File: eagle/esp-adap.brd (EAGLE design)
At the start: 26.5 x 11.2 mm, 3 parts

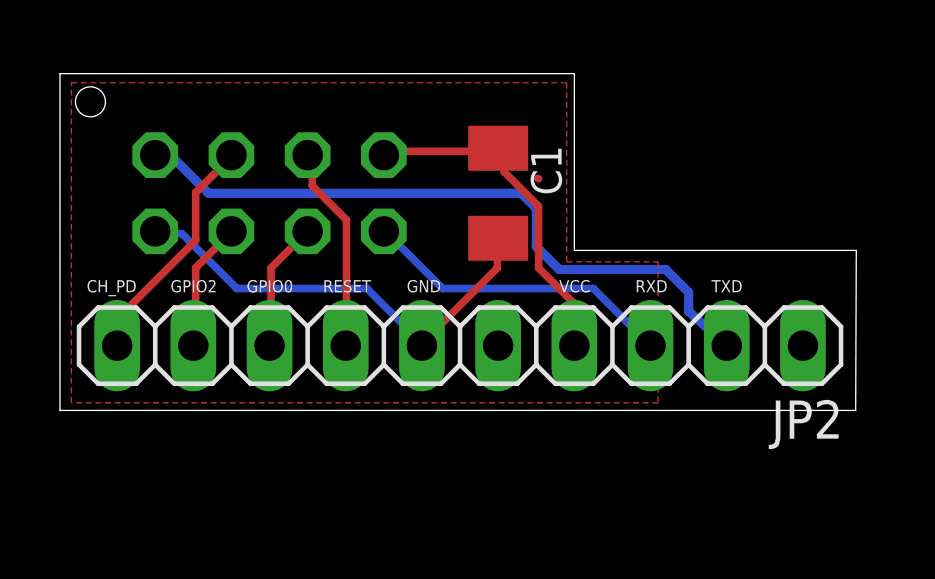
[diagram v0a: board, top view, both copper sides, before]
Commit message: added docs
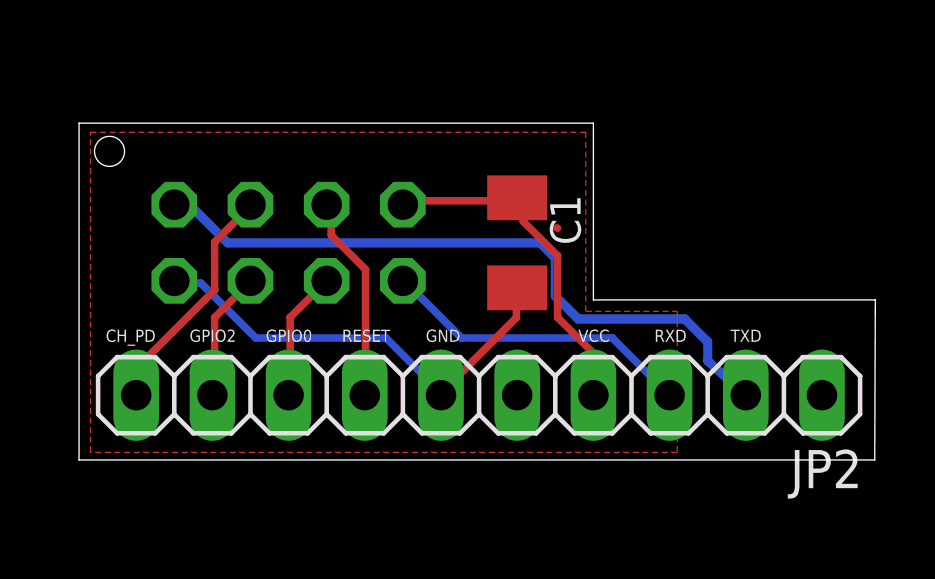
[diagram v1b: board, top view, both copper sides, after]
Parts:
- moved JP1 1.77 mm to (6.99, 7.24)
- moved JP2 1.77 mm to (13.3, 2.16)
- moved C1 1.77 mm to (14.6, 7.24)

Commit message: redefined board
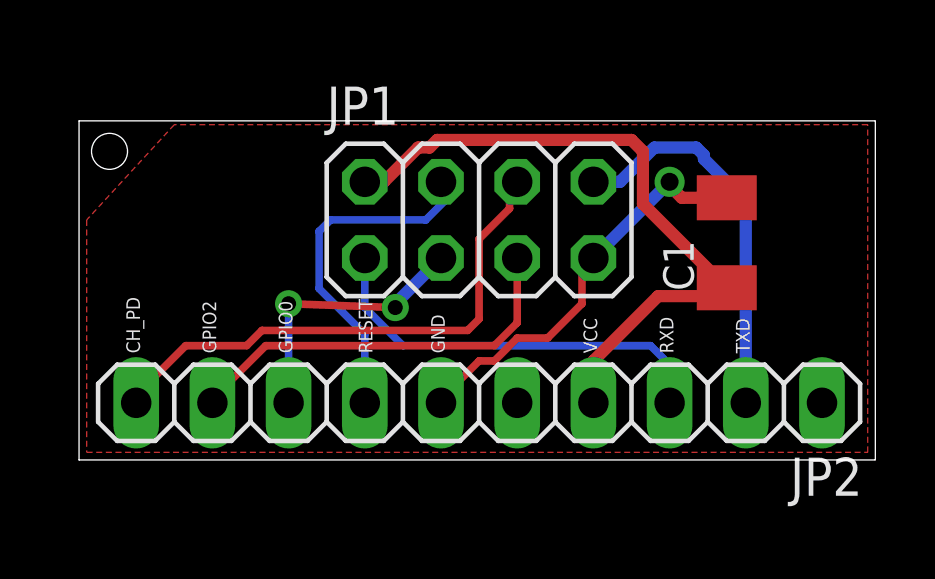
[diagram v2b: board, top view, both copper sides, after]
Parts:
- moved C1 6.98 mm to (21.6, 7.24), turned to 90 degrees
- moved JP1 6.40 mm to (13.3, 8.00), flipped to the top
- moved JP2 0.25 mm to (13.3, 1.91)
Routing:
- net VCC: track 11.6 -> 22.6 mm
- net CH_PD: track 7.93 -> 17.8 mm
- net TXD: track 22.8 -> 13.1 mm
- net GPIO2: track 4.33 -> 13.5 mm
- net GPIO0: track 4.33 -> 9.14 mm, vias 0 -> 2
- net RESET: track 6.91 -> 11.6 mm
- net RXD: track 10.5 -> 13.9 mm
- net GND: track 15.1 -> 13.6 mm, vias 0 -> 1
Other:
- board size 26.5 x 11.2 mm -> 26.5 x 11.3 mm

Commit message: changed header
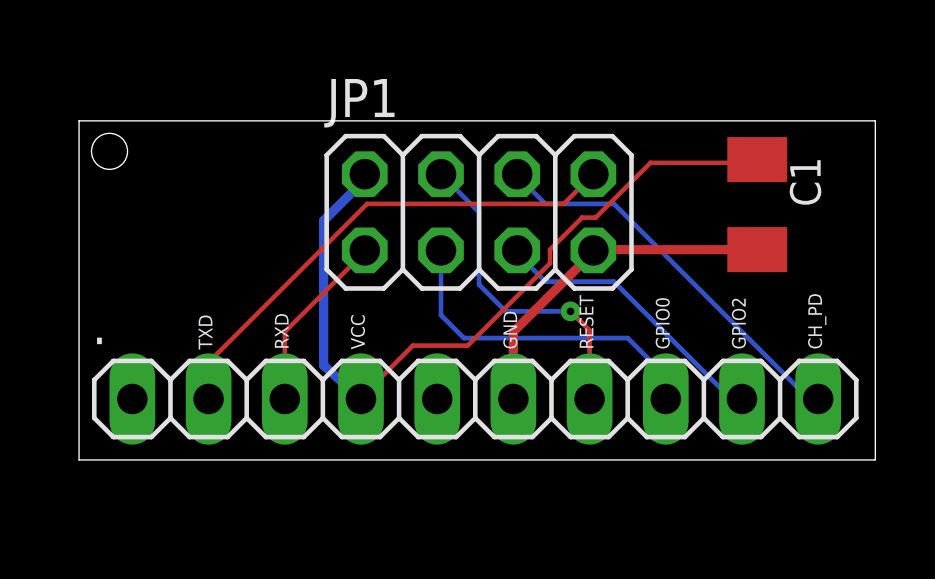
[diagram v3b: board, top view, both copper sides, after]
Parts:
- removed JP2: (no value), pinhead:1X10
- added .: (no value), pinhead:1X10
- moved C1 1.63 mm to (22.6, 8.51), turned to 270 degrees
- moved JP1 0.25 mm to (13.3, 8.26)
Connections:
- net CH_PD: now also ..10; no longer JP2.10
- net GND: now also ..6; no longer JP2.6
- net GPIO0: now also ..8; no longer JP2.8
- net GPIO2: now also ..9; no longer JP2.9
- net RESET: now also ..7; no longer JP2.7
- net RXD: now also ..3; no longer JP2.3
- net TXD: now also ..2; no longer JP2.2
- net VCC: now also ..4; no longer JP2.4
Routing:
- net RXD: track 13.9 -> 6.05 mm
- net CH_PD: track 17.8 -> 13.2 mm
- net GPIO2: track 13.5 -> 9.66 mm
- net TXD: track 13.1 -> 16.6 mm
- net VCC: track 22.6 -> 25.4 mm
- net GND: track 13.6 -> 11.5 mm, vias 1 -> 0
- net GPIO0: track 9.14 -> 11.3 mm, vias 2 -> 0
- net RESET: track 11.6 -> 10.8 mm, vias 0 -> 1
- removed copper zone on layer 1, net VCC
